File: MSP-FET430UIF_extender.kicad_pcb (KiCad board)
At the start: 2 copper layers, 8 parts, among them P1 CONN_01X03, P2 CONN_02X07, P3 CONN_01X02, P4 CONN_01X08

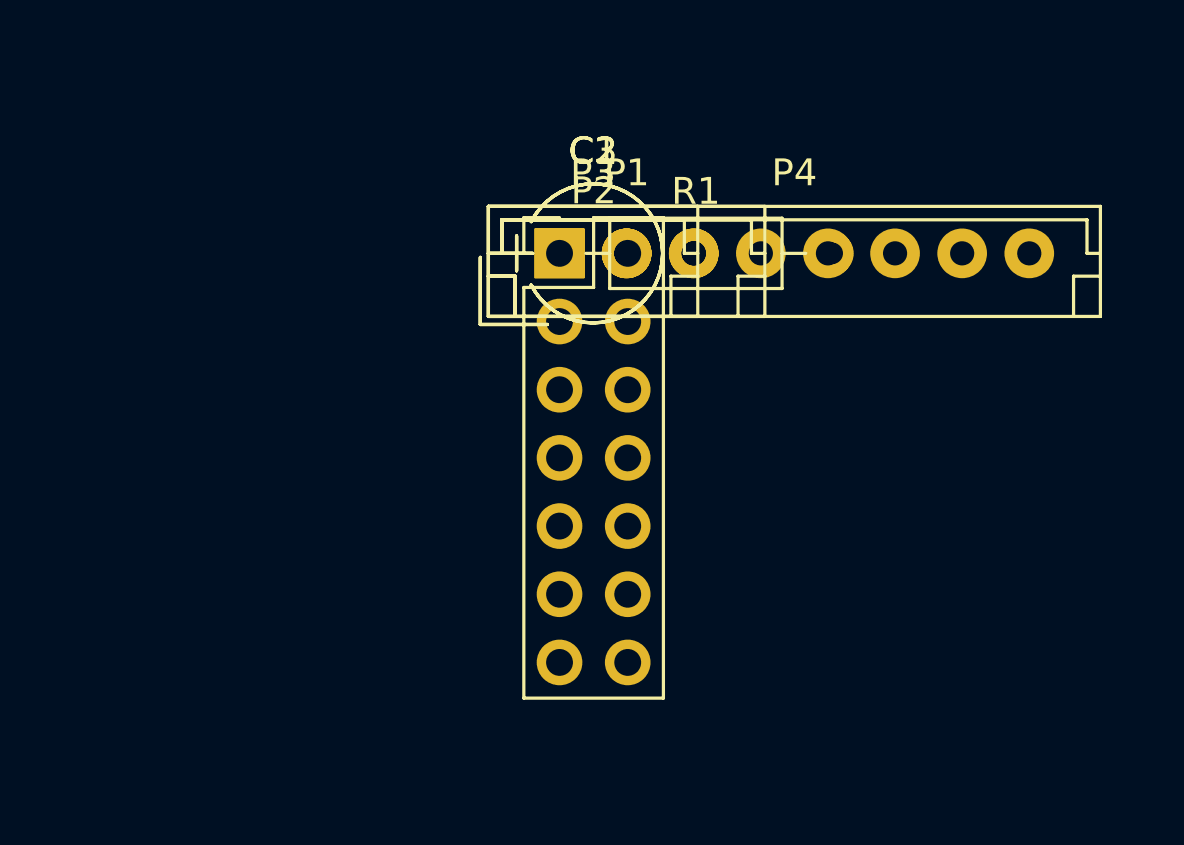
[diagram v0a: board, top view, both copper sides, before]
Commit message: *finalized pcb layout
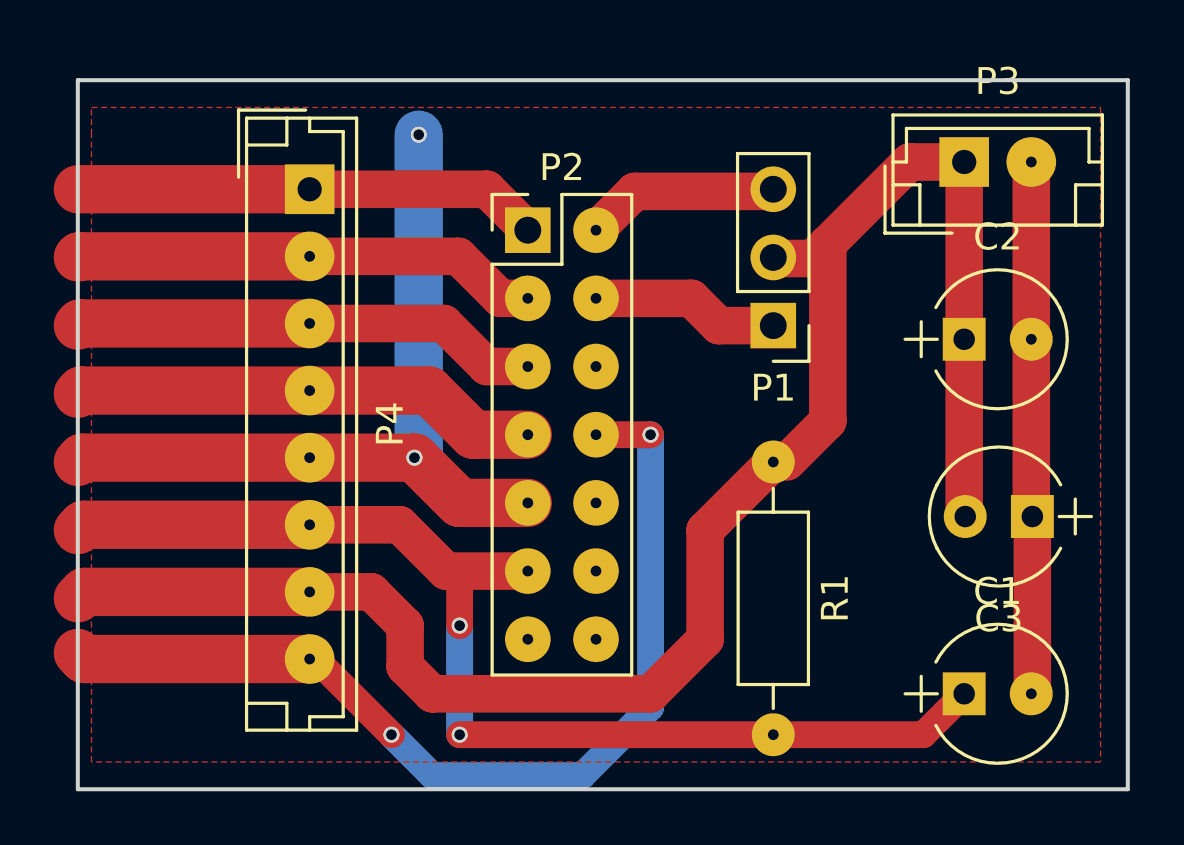
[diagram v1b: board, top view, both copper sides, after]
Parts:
- P1: footprint Connectors_JST:JST_EH_B03B-EH-A_03x2.50mm_Straight -> Pin_Headers:Pin_Header_Straight_1x03_Pitch2.54mm
- moved C1 22.3 mm to (163.6, 121.4)
- moved C3 20.2 mm to (166.1, 114.8), turned to 180 degrees
- moved P3 15.5 mm to (163.6, 101.6)
- moved C2 15.4 mm to (163.6, 108.2)
- moved R1 11.1 mm to (156.5, 112.8), turned to 270 degrees
- moved P4 9.61 mm to (139.2, 102.6), turned to 270 degrees
- moved P1 8.41 mm to (156.5, 107.7), turned to 180 degrees
- moved P2 1.46 mm to (147.3, 104.1)
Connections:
- C2 pad 2: Net-(C2-Pad2) -> /GND
- C3 pad 1: Net-(C2-Pad2) -> /GND
- P3 pad 2: Net-(C2-Pad2) -> /GND
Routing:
- net /VCC: track 0.00 -> 65.5 mm
- net /GND: track 0.00 -> 51.9 mm, vias 0 -> 2
- net /RST: track 0.00 -> 45.6 mm, vias 0 -> 2
- net /TEST: track 0.00 -> 36.5 mm, vias 0 -> 2
- net /TCK: track 0.00 -> 17.5 mm
- net /TMS: track 0.00 -> 17.5 mm
- net /TDI: track 0.00 -> 17.4 mm
- net /TDO: track 0.00 -> 17.4 mm
- net /VCC_TOOL: track 0.00 -> 7.20 mm
- net /VCC_TARGET: track 0.00 -> 7.02 mm
- added copper zone on F.Cu, net /GND
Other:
- board outline added: 39.1 x 26.4 mm
